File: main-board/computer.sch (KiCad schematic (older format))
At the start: 26 parts, among them J1 Conn_02x20_Odd_Even, J2 Conn_02x20_Odd_Even, J3 PORT A, J4 PORT B, J5 SERIAL, SW1 RESET, U1 W65C02S, U11 DS1813, U2 AS6C62256-55, U3 SST39SF010, U4 W65C22N, U5 W65C51N, U6 74HC00, U7 74HC30, U8 74HC138, X1 1.8432MHz

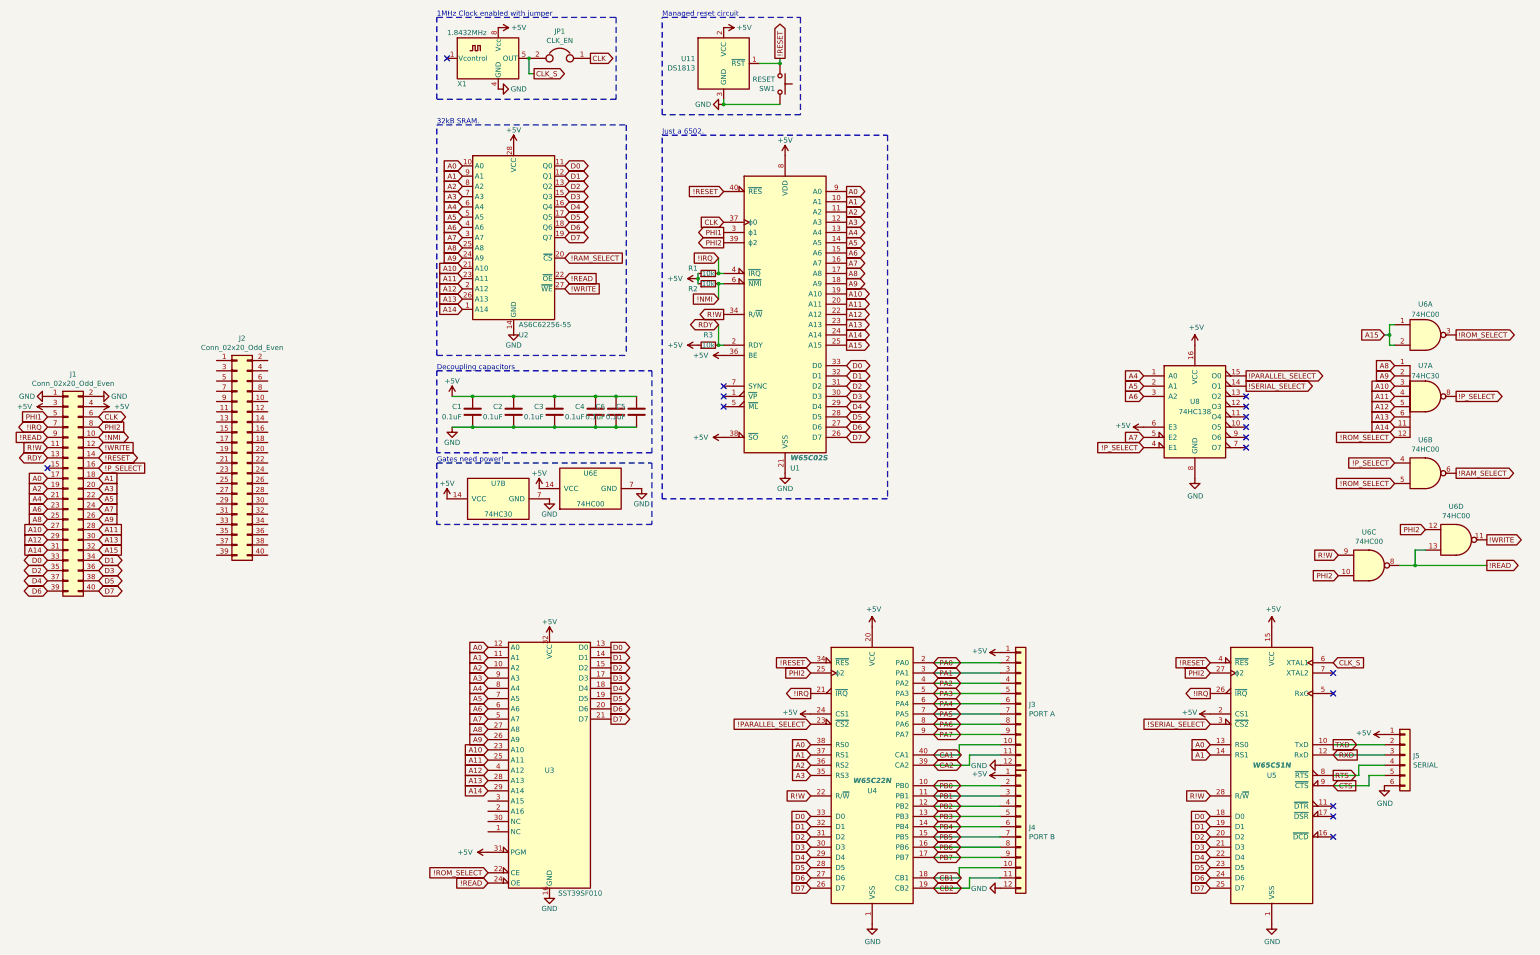
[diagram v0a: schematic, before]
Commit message: Revert "Integtrate IO into mail board, begion VGA layout"
This reverts commit 15baf3f71fbe492a9e0b6e5b5ec863db56e31855.
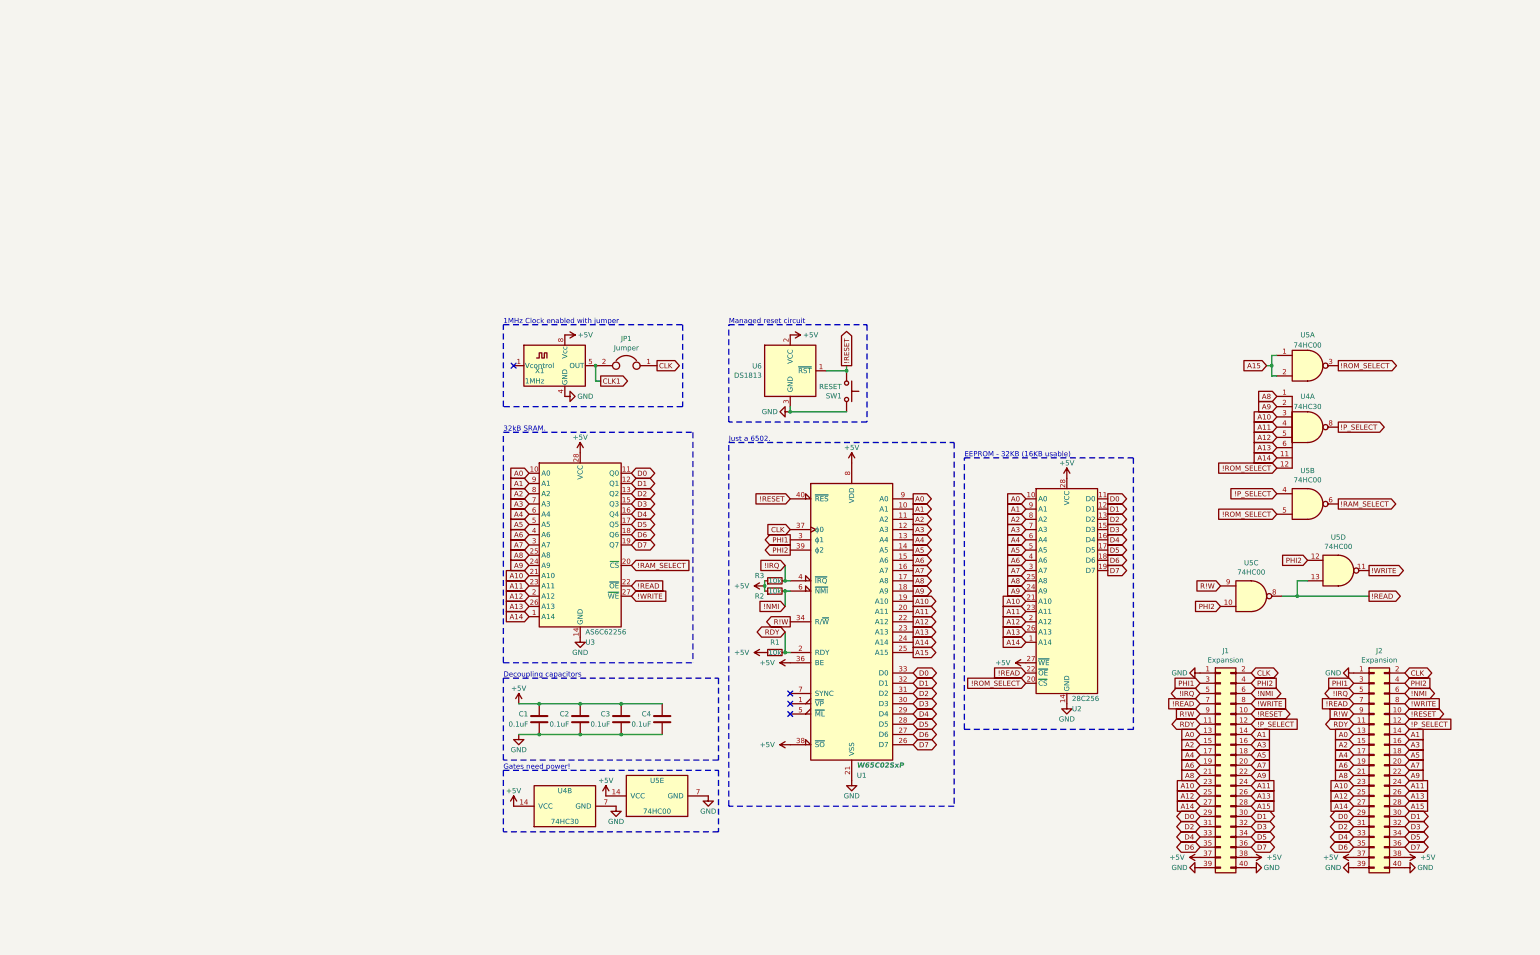
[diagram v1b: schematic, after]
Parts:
- removed C5, C6: 0.1uF, Capacitor_THT:C_Disc_D6.0mm_W2.5mm_P5.00mm, symbol Device:C
- removed J3: PORT A, Connector_PinHeader_2.54mm:PinHeader_1x12_P2.54mm_Horizontal, symbol Connector_Generic:Conn_01x12
- removed J4: PORT B, Connector_PinHeader_2.54mm:PinHeader_1x12_P2.54mm_Horizontal, symbol Connector_Generic:Conn_01x12
- removed J5: SERIAL, Connector_PinHeader_2.54mm:PinHeader_1x06_P2.54mm_Horizontal, symbol Connector_Generic:Conn_01x06
- removed U3: SST39SF010, Package_DIP:DIP-32_W15.24mm_Socket, symbol computer:SST39SF010
- removed U4: W65C22N, Package_DIP:DIP-40_W15.24mm_Socket, symbol 65xx:W65C22NxP
- removed U5: W65C51N, Package_DIP:DIP-28_W15.24mm_Socket, symbol 65xx:W65C51NxP
- removed U8: 74HC138, Package_DIP:DIP-16_W7.62mm_Socket, symbol 74xx:74LS138
- added U2: 28C256, Package_DIP:DIP-28_W15.24mm_Socket, symbol Memory_EEPROM:28C256
- J1, J2: value Conn_02x20_Odd_Even -> Expansion; footprint Connector_PinSocket_2.54mm:PinSocket_2x20_P2.54mm_Vertical -> Connector_PinHeader_2.54mm:PinHeader_2x20_P2.54mm_Vertical
- JP1: value CLK_EN -> Jumper
- U1: value W65C02S -> W65C02SxP
- U3: renamed from U2; value AS6C62256-55 -> AS6C62256
- U5: renamed from U6; footprint Package_DIP:DIP-14_W7.62mm_Socket -> (none)
- X1: value 1.8432MHz -> 1MHz
- renumbered R3 to R1, R1 to R3, U7 to U4, U6 to U5, U11 to U6
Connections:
- net !IRQ: now also J1.5 (Pin_5), J2.5 (Pin_5); no longer J1.7 (Pin_7)
- net !NMI: now also J1.6 (Pin_6), J2.6 (Pin_6); no longer J1.10 (Pin_10)
- net !P_SELECT: now also J1.12 (Pin_12), J2.12 (Pin_12); no longer J1.16 (Pin_16)
- net !READ: now also J1.7 (Pin_7), J2.7 (Pin_7), U2.22 (~OE); no longer J1.9 (Pin_9)
- net !RESET: now also J1.10 (Pin_10), J2.10 (Pin_10); no longer J1.14 (Pin_14)
- net !ROM_SELECT: now also U2.20 (~CS)
- net !WRITE: now also J1.8 (Pin_8), J2.8 (Pin_8); no longer J1.12 (Pin_12)
- net +5V: now also J1.37 (Pin_37), J1.38 (Pin_38), J2.37 (Pin_37), J2.38 (Pin_38), U2.27 (~WE), U2.28 (VCC); no longer J1.3 (Pin_3), J1.4 (Pin_4)
- net A0: now also J1.13 (Pin_13), J2.13 (Pin_13), U2.10 (A0); no longer J1.17 (Pin_17)
- net A1: now also J1.14 (Pin_14), J2.14 (Pin_14), U2.9 (A1); no longer J1.18 (Pin_18)
- net A10: now also J1.23 (Pin_23), J2.23 (Pin_23), U2.21 (A10); no longer J1.27 (Pin_27)
- net A11: now also J1.24 (Pin_24), J2.24 (Pin_24), U2.23 (A11); no longer J1.28 (Pin_28)
- net A12: now also J1.25 (Pin_25), J2.25 (Pin_25), U2.2 (A12); no longer J1.29 (Pin_29)
- net A13: now also J1.26 (Pin_26), J2.26 (Pin_26), U2.26 (A13); no longer J1.30 (Pin_30)
- net A14: now also J1.27 (Pin_27), J2.27 (Pin_27), U2.1 (A14); no longer J1.31 (Pin_31)
- net A15: now also J1.28 (Pin_28), J2.28 (Pin_28); no longer J1.32 (Pin_32)
- net A2: now also J1.15 (Pin_15), J2.15 (Pin_15), U2.8 (A2); no longer J1.19 (Pin_19)
- net A3: now also J1.16 (Pin_16), J2.16 (Pin_16), U2.7 (A3); no longer J1.20 (Pin_20)
- net A4: now also J1.17 (Pin_17), J2.17 (Pin_17), U2.6 (A4); no longer J1.21 (Pin_21)
- net A5: now also J1.18 (Pin_18), J2.18 (Pin_18), U2.5 (A5); no longer J1.22 (Pin_22)
- net A6: now also J1.19 (Pin_19), J2.19 (Pin_19), U2.4 (A6); no longer J1.23 (Pin_23)
- net A7: now also J1.20 (Pin_20), J2.20 (Pin_20), U2.3 (A7); no longer J1.24 (Pin_24)
- net A8: now also J1.21 (Pin_21), J2.21 (Pin_21), U2.25 (A8); no longer J1.25 (Pin_25)
- net A9: now also J1.22 (Pin_22), J2.22 (Pin_22), U2.24 (A9); no longer J1.26 (Pin_26)
- net CLK: now also J1.2 (Pin_2), J2.2 (Pin_2); no longer J1.6 (Pin_6)
- net D0: now also J1.29 (Pin_29), J2.29 (Pin_29), U2.11 (D0); no longer J1.33 (Pin_33)
- net D1: now also J1.30 (Pin_30), J2.30 (Pin_30), U2.12 (D1); no longer J1.34 (Pin_34)
- net D2: now also J1.31 (Pin_31), J2.31 (Pin_31), U2.13 (D2); no longer J1.35 (Pin_35)
- net D3: now also J1.32 (Pin_32), J2.32 (Pin_32), U2.15 (D3); no longer J1.36 (Pin_36)
- net D4: now also J1.33 (Pin_33), J2.33 (Pin_33), U2.16 (D4); no longer J1.37 (Pin_37)
- net D5: now also J1.34 (Pin_34), J2.34 (Pin_34), U2.17 (D5); no longer J1.38 (Pin_38)
- net D6: now also J1.35 (Pin_35), J2.35 (Pin_35), U2.18 (D6); no longer J1.39 (Pin_39)
- net D7: now also J1.36 (Pin_36), J2.36 (Pin_36), U2.19 (D7); no longer J1.40 (Pin_40)
- net GND: now also J1.39 (Pin_39), J1.40 (Pin_40), J2.1 (Pin_1), J2.39 (Pin_39), J2.40 (Pin_40), U2.14 (GND); no longer J1.2 (Pin_2)
- net PHI1: now also J1.3 (Pin_3), J2.3 (Pin_3); no longer J1.5 (Pin_5)
- net PHI2: now also J1.4 (Pin_4), J2.4 (Pin_4); no longer J1.8 (Pin_8)
- net R!W: now also J1.9 (Pin_9), J2.9 (Pin_9); no longer J1.11 (Pin_11)
- net RDY: now also J1.11 (Pin_11), J2.11 (Pin_11); no longer J1.13 (Pin_13)
- net CLK_S renamed CLK1
- no-connect marks 16 -> 4
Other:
- note added: "EEPROM - 32KB (16KB usable)"
- moved on the sheet: C1, C2, JP1, R1, R2, R3, SW1, U1, U3, U4A, U4B, U5A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

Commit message: Integtrate IO into mail board, begion VGA layout
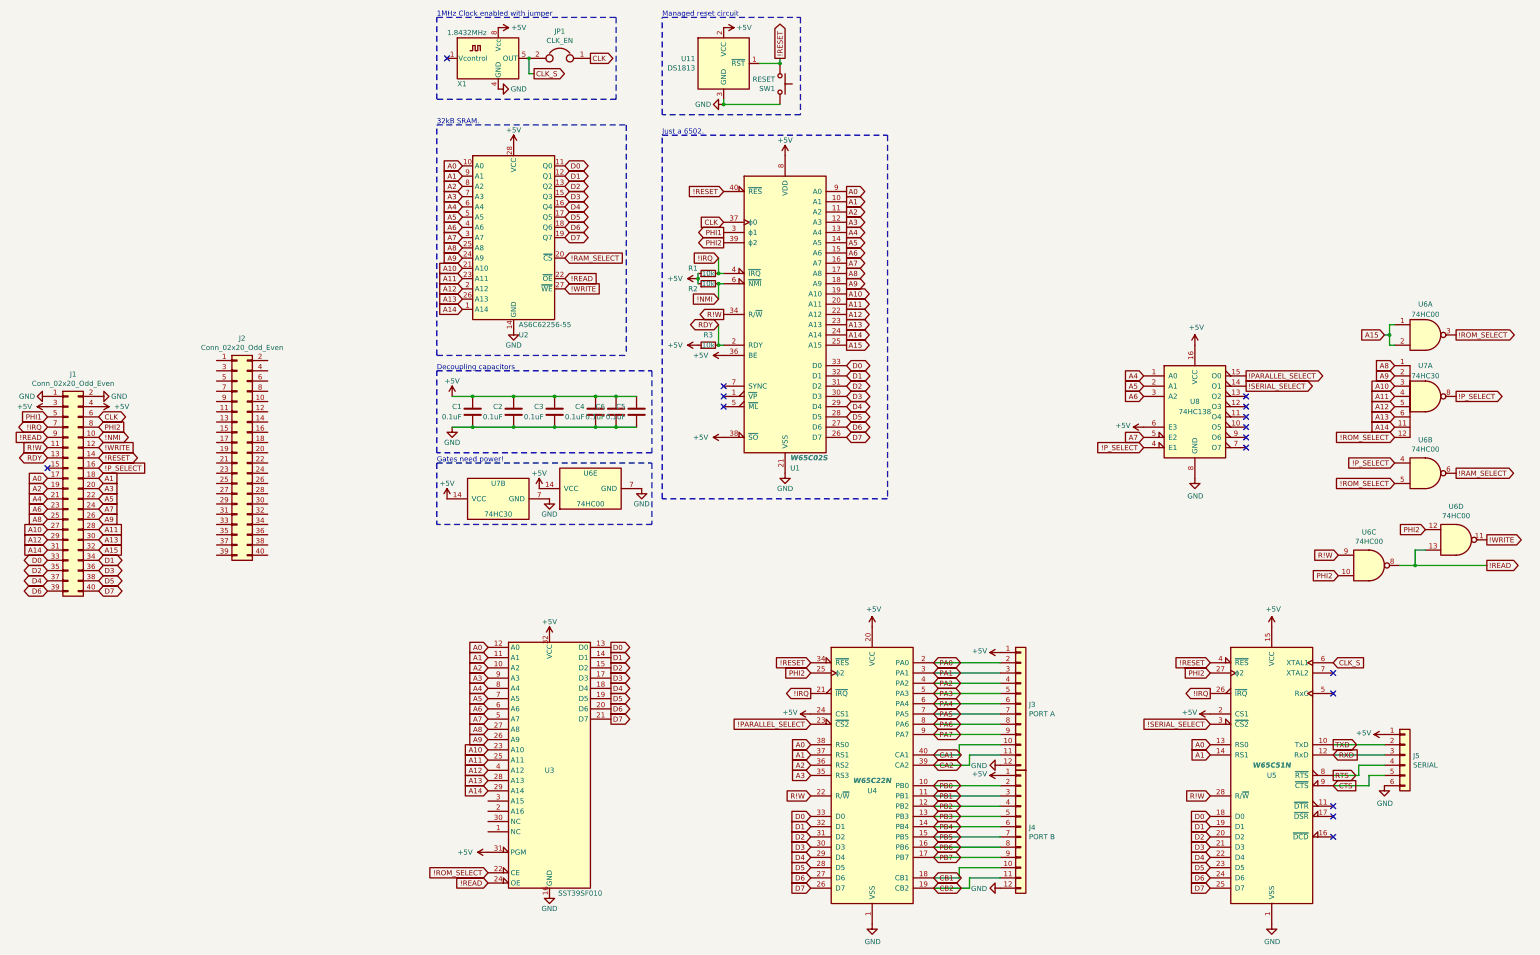
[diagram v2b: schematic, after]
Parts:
- removed U2: 28C256, Package_DIP:DIP-28_W15.24mm_Socket, symbol Memory_EEPROM:28C256
- added C5, C6: 0.1uF, Capacitor_THT:C_Disc_D6.0mm_W2.5mm_P5.00mm, symbol Device:C
- added J3: PORT A, Connector_PinHeader_2.54mm:PinHeader_1x12_P2.54mm_Horizontal, symbol Connector_Generic:Conn_01x12
- added J4: PORT B, Connector_PinHeader_2.54mm:PinHeader_1x12_P2.54mm_Horizontal, symbol Connector_Generic:Conn_01x12
- added J5: SERIAL, Connector_PinHeader_2.54mm:PinHeader_1x06_P2.54mm_Horizontal, symbol Connector_Generic:Conn_01x06
- added U3: SST39SF010, Package_DIP:DIP-32_W15.24mm_Socket, symbol computer:SST39SF010
- added U4: W65C22N, Package_DIP:DIP-40_W15.24mm_Socket, symbol 65xx:W65C22NxP
- added U5: W65C51N, Package_DIP:DIP-28_W15.24mm_Socket, symbol 65xx:W65C51NxP
- added U8: 74HC138, Package_DIP:DIP-16_W7.62mm_Socket, symbol 74xx:74LS138
- J1, J2: value Expansion -> Conn_02x20_Odd_Even; footprint Connector_PinHeader_2.54mm:PinHeader_2x20_P2.54mm_Vertical -> Connector_PinSocket_2.54mm:PinSocket_2x20_P2.54mm_Vertical
- JP1: value Jumper -> CLK_EN
- U1: value W65C02SxP -> W65C02S
- U2: renamed from U3; value AS6C62256 -> AS6C62256-55
- U6: renamed from U5; footprint (none) -> Package_DIP:DIP-14_W7.62mm_Socket
- X1: value 1MHz -> 1.8432MHz
- renumbered R3 to R1, R1 to R3, U6 to U11, U5 to U6, U4 to U7
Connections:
- net !IRQ: now also J1.7 (Pin_7), U4.21 (~IRQ), U5.26 (~IRQ); no longer J1.5 (Pin_5), J2.5 (Pin_5)
- net !NMI: now also J1.10 (Pin_10); no longer J1.6 (Pin_6), J2.6 (Pin_6)
- net !P_SELECT: now also J1.16 (Pin_16), U8.4 (E1); no longer J1.12 (Pin_12), J2.12 (Pin_12)
- net !READ: now also J1.9 (Pin_9), U3.24 (OE); no longer J1.7 (Pin_7), J2.7 (Pin_7)
- net !RESET: now also J1.14 (Pin_14), U4.34 (~RES), U5.4 (~RES); no longer J1.10 (Pin_10), J2.10 (Pin_10)
- net !ROM_SELECT: now also U3.22 (CE)
- net !WRITE: now also J1.12 (Pin_12); no longer J1.8 (Pin_8), J2.8 (Pin_8)
- net +5V: now also J1.3 (Pin_3), J1.4 (Pin_4), C5.1, C6.1, J3.1 (Pin_1), J4.1 (Pin_1), J5.1 (Pin_1), U3.31 (PGM), U3.32 (VCC), U4.20 (VCC), U4.24 (CS1), U5.15 (VCC), U5.2 (CS1), U8.16 (VCC), U8.6 (E3); no longer J1.37 (Pin_37), J1.38 (Pin_38), J2.37 (Pin_37), J2.38 (Pin_38)
- net A0: now also J1.17 (Pin_17), U3.12 (A0), U4.38 (RS0), U5.13 (RS0); no longer J1.13 (Pin_13), J2.13 (Pin_13)
- net A1: now also J1.18 (Pin_18), U3.11 (A1), U4.37 (RS1), U5.14 (RS1); no longer J1.14 (Pin_14), J2.14 (Pin_14)
- net A10: now also J1.27 (Pin_27), U3.23 (A10); no longer J1.23 (Pin_23), J2.23 (Pin_23)
- net A11: now also J1.28 (Pin_28), U3.25 (A11); no longer J1.24 (Pin_24), J2.24 (Pin_24)
- net A12: now also J1.29 (Pin_29), U3.4 (A12); no longer J1.25 (Pin_25), J2.25 (Pin_25)
- net A13: now also J1.30 (Pin_30), U3.28 (A13); no longer J1.26 (Pin_26), J2.26 (Pin_26)
- net A14: now also J1.31 (Pin_31), U3.29 (A14); no longer J1.27 (Pin_27), J2.27 (Pin_27)
- net A15: now also J1.32 (Pin_32); no longer J1.28 (Pin_28), J2.28 (Pin_28)
- net A2: now also J1.19 (Pin_19), U3.10 (A2), U4.36 (RS2); no longer J1.15 (Pin_15), J2.15 (Pin_15)
- net A3: now also J1.20 (Pin_20), U3.9 (A3), U4.35 (RS3); no longer J1.16 (Pin_16), J2.16 (Pin_16)
- net A4: now also J1.21 (Pin_21), U3.8 (A4), U8.1 (A0); no longer J1.17 (Pin_17), J2.17 (Pin_17)
- net A5: now also J1.22 (Pin_22), U3.7 (A5), U8.2 (A1); no longer J1.18 (Pin_18), J2.18 (Pin_18)
- net A6: now also J1.23 (Pin_23), U3.6 (A6), U8.3 (A2); no longer J1.19 (Pin_19), J2.19 (Pin_19)
- net A7: now also J1.24 (Pin_24), U3.5 (A7), U8.5 (E2); no longer J1.20 (Pin_20), J2.20 (Pin_20)
- net A8: now also J1.25 (Pin_25), U3.27 (A8); no longer J1.21 (Pin_21), J2.21 (Pin_21)
- net A9: now also J1.26 (Pin_26), U3.26 (A9); no longer J1.22 (Pin_22), J2.22 (Pin_22)
- net CLK: now also J1.6 (Pin_6); no longer J1.2 (Pin_2), J2.2 (Pin_2)
- net D0: now also J1.33 (Pin_33), U3.13 (D0), U4.33 (D0), U5.18 (D0); no longer J1.29 (Pin_29), J2.29 (Pin_29)
- net D1: now also J1.34 (Pin_34), U3.14 (D1), U4.32 (D1), U5.19 (D1); no longer J1.30 (Pin_30), J2.30 (Pin_30)
- net D2: now also J1.35 (Pin_35), U3.15 (D2), U4.31 (D2), U5.20 (D2); no longer J1.31 (Pin_31), J2.31 (Pin_31)
- net D3: now also J1.36 (Pin_36), U3.17 (D3), U4.30 (D3), U5.21 (D3); no longer J1.32 (Pin_32), J2.32 (Pin_32)
- net D4: now also J1.37 (Pin_37), U3.18 (D4), U4.29 (D4), U5.22 (D4); no longer J1.33 (Pin_33), J2.33 (Pin_33)
- net D5: now also J1.38 (Pin_38), U3.19 (D5), U4.28 (D5), U5.23 (D5); no longer J1.34 (Pin_34), J2.34 (Pin_34)
- net D6: now also J1.39 (Pin_39), U3.20 (D6), U4.27 (D6), U5.24 (D6); no longer J1.35 (Pin_35), J2.35 (Pin_35)
- net D7: now also J1.40 (Pin_40), U3.21 (D7), U4.26 (D7), U5.25 (D7); no longer J1.36 (Pin_36), J2.36 (Pin_36)
- net GND: now also J1.2 (Pin_2), C5.2, C6.2, J3.12 (Pin_12), J4.12 (Pin_12), J5.6 (Pin_6), U3.16 (GND), U4.1 (VSS), U5.1 (VSS), U8.8 (GND); no longer J1.39 (Pin_39), J1.40 (Pin_40), J2.1 (Pin_1), J2.39 (Pin_39), J2.40 (Pin_40)
- net PHI1: now also J1.5 (Pin_5); no longer J1.3 (Pin_3), J2.3 (Pin_3)
- net PHI2: now also J1.8 (Pin_8), U4.25 (ϕ2), U5.27 (ϕ2); no longer J1.4 (Pin_4), J2.4 (Pin_4)
- net R!W: now also J1.11 (Pin_11), U4.22 (R/~W), U5.28 (R/~W); no longer J1.9 (Pin_9), J2.9 (Pin_9)
- net RDY: now also J1.13 (Pin_13); no longer J1.11 (Pin_11), J2.11 (Pin_11)
- net CLK1 renamed CLK_S
- net CLK_S: now also U5.6 (XTAL1)
- new net !PARALLEL_SELECT: U4.23 (~CS2), U8.15 (O0)
- new net !SERIAL_SELECT: U5.3 (~CS2), U8.14 (O1)
- new net CA1: J3.10 (Pin_10), U4.40 (CA1)
- new net CA2: J3.11 (Pin_11), U4.39 (CA2)
- new net CB1: J4.10 (Pin_10), U4.18 (CB1)
- new net CB2: J4.11 (Pin_11), U4.19 (CB2)
- new net CTS: J5.5 (Pin_5), U5.9 (~CTS)
- new net PA0: J3.2 (Pin_2), U4.2 (PA0)
- new net PA1: J3.3 (Pin_3), U4.3 (PA1)
- new net PA2: J3.4 (Pin_4), U4.4 (PA2)
- new net PA3: J3.5 (Pin_5), U4.5 (PA3)
- new net PA4: J3.6 (Pin_6), U4.6 (PA4)
- new net PA5: J3.7 (Pin_7), U4.7 (PA5)
- new net PA6: J3.8 (Pin_8), U4.8 (PA6)
- new net PA7: J3.9 (Pin_9), U4.9 (PA7)
- new net PB0: J4.2 (Pin_2), U4.10 (PB0)
- new net PB1: J4.3 (Pin_3), U4.11 (PB1)
- new net PB2: J4.4 (Pin_4), U4.12 (PB2)
- new net PB3: J4.5 (Pin_5), U4.13 (PB3)
- new net PB4: J4.6 (Pin_6), U4.14 (PB4)
- new net PB5: J4.7 (Pin_7), U4.15 (PB5)
- new net PB6: J4.8 (Pin_8), U4.16 (PB6)
- new net PB7: J4.9 (Pin_9), U4.17 (PB7)
- new net RTS: J5.4 (Pin_4), U5.8 (~RTS)
- new net RXD: J5.3 (Pin_3), U5.12 (RxD)
- new net TXD: J5.2 (Pin_2), U5.10 (TxD)
- no-connect marks 4 -> 16
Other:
- note removed: "EEPROM - 32KB (16KB usable)"
- moved on the sheet: C1, C2, JP1, R1, R2, R3, SW1, U1, U11, U2, U6A, U6B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
